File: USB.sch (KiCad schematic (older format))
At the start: 4 parts, among them J2 USB_B_Micro, U2 USBLC6-2SC6

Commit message: a
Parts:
- C15: footprint (none) -> Capacitor_SMD:C_0603_1608Metric
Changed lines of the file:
@@
 F 0 "C15" H 5365 3296 50  0000 L CNN
 F 1 "C" H 5365 3205 50  0000 L CNN
-F 2 "" H 5288 3100 50  0001 C CNN
+F 2 "Capacitor_SMD:C_0603_1608Metric" H 5288 3100 50  0001 C CNN
 F 3 "~" H 5250 3250 50  0001 C CNN
 	1    5250 3250

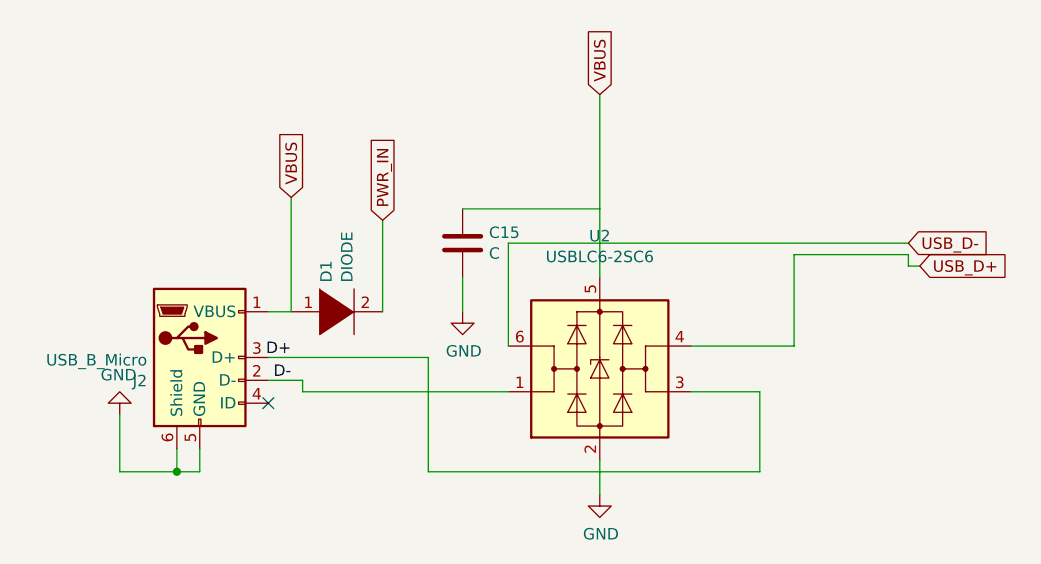
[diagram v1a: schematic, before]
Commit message: finish board
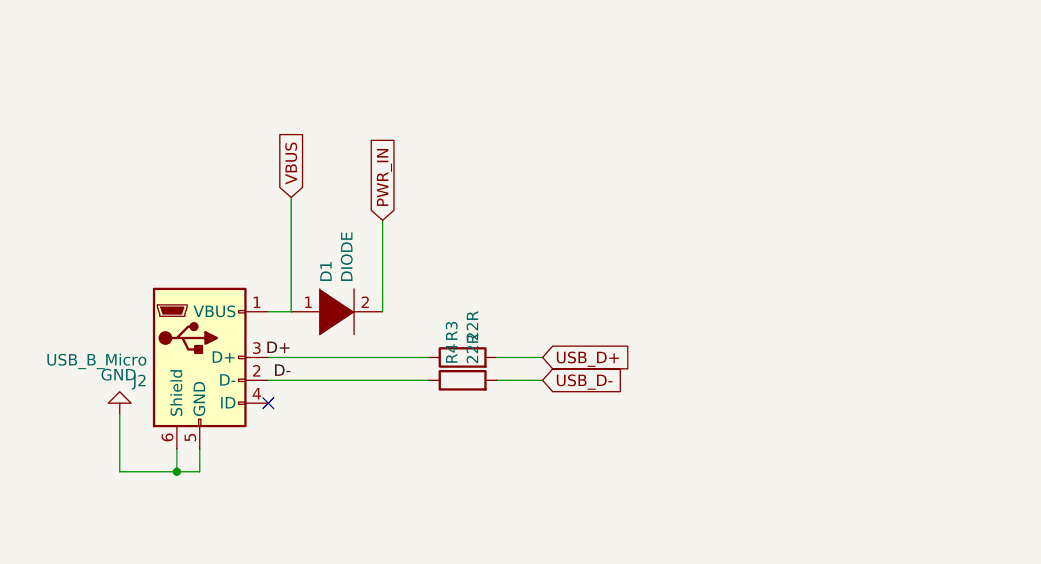
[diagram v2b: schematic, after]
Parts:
- removed C15: C, Capacitor_SMD:C_0603_1608Metric, symbol Device:C
- removed U2: USBLC6-2SC6, Package_TO_SOT_SMD:SOT-23-6, symbol Power_Protection:USBLC6-2SC6
- added R3, R4: 22R, Resistor_SMD:R_0603_1608Metric_Pad1.05x0.95mm_HandSolder, symbol Device:R
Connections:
- net D+: now also R3.1
- net D-: now also R4.1
- net USB_D+: now also R3.2
- net USB_D-: now also R4.2
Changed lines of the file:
@@
 Comment4 ""
 $EndDescr
-$Comp
-L Power_Protection:USBLC6-2SC6 U?
-U 1 1 5F5427BF
-P 5850 3800
-AR Path="/5F5427BF" Ref="U?"  Part="1"
-AR Path="/5F2F6324/5F5427BF" Ref="U?"  Part="1"
-AR Path="/5F53A524/5F5427BF" Ref="U2"  Part="1"
-AR Path="/5F584BC5/5F5427BF" Ref="U?"  Part="1"
-AR Path="/5FD47887/5F5427BF" Ref="U?"  Part="1"
-F 0 "U2" H 5850 4381 50  0000 C CNN
-F 1 "USBLC6-2SC6" H 5850 4290 50  0000 C CNN
-F 2 "Package_TO_SOT_SMD:SOT-23-6" H 5850 3300 50  0001 C CNN
-F 3 "https://www.st.com/resource/en/datasheet/usblc6-2.pdf" H 6050 4150 50  0001 C CNN
-	1    5850 3800
-	1    0    0    -1
-$EndComp
 Wire Wire Line
 	4100 4150 4100 4250
@@
 $EndComp
 NoConn ~ 4400 3950
-Wire Wire Line
-	4550 3850 4550 3900
-Wire Wire Line
-	4550 3850 4400 3850
 Text Label 4500 3750 2    50   ~ 0
 D+
@@
 D-
 Wire Wire Line
-	4550 3900 5450 3900
-Wire Wire Line
-	5100 3750 5100 4250
-Wire Wire Line
-	5100 4250 6550 4250
-Wire Wire Line
-	6550 4250 6550 3900
-Wire Wire Line
-	6550 3900 6250 3900
-Wire Wire Line
 	4400 3750 5100 3750
-Wire Wire Line
-	6250 3700 6700 3700
-Wire Wire Line
-	6700 3700 6700 3300
-Wire Wire Line
-	6700 3300 7200 3300
-Wire Wire Line
-	5450 3700 5450 3250
-Wire Wire Line
-	5450 3250 7200 3250
-Wire Wire Line
-	5850 3400 5850 3100
-Wire Wire Line
-	5850 4200 5850 4350
-$Comp
-L power:GND #PWR?
-U 1 1 5F5427E0
-P 5850 4350
-AR Path="/5F2F6324/5F5427E0" Ref="#PWR?"  Part="1"
-AR Path="/5F5427E0" Ref="#PWR?"  Part="1"
-AR Path="/5F53A524/5F5427E0" Ref="#PWR0112"  Part="1"
-AR Path="/5F584BC5/5F5427E0" Ref="#PWR?"  Part="1"
-AR Path="/5FD47887/5F5427E0" Ref="#PWR?"  Part="1"
-F 0 "#PWR0112" H 5850 4100 50  0001 C CNN
-F 1 "GND" H 5855 4177 50  0000 C CNN
-F 2 "" H 5850 4350 50  0001 C CNN
-F 3 "" H 5850 4350 50  0001 C CNN
-	1    5850 4350
-	1    0    0    -1
-$EndComp
-Wire Wire Line
-	7250 3350 7200 3350
-Wire Wire Line
-	7200 3350 7200 3300
-$Comp
-L Device:C C?
-U 1 1 5F5427E8
-P 5250 3250
-AR Path="/5F2F6324/5F5427E8" Ref="C?"  Part="1"
-AR Path="/5F5427E8" Ref="C?"  Part="1"
-AR Path="/5F53A524/5F5427E8" Ref="C15"  Part="1"
-AR Path="/5F584BC5/5F5427E8" Ref="C?"  Part="1"
-AR Path="/5FD47887/5F5427E8" Ref="C?"  Part="1"
-F 0 "C15" H 5365 3296 50  0000 L CNN
-F 1 "C" H 5365 3205 50  0000 L CNN
-F 2 "Capacitor_SMD:C_0603_1608Metric" H 5288 3100 50  0001 C CNN
-F 3 "~" H 5250 3250 50  0001 C CNN
-	1    5250 3250
-	1    0    0    -1
-$EndComp
-Wire Wire Line
-	5250 3100 5850 3100
-Wire Wire Line
-	5250 3400 5250 3550
-$Comp
-L power:GND #PWR?
-U 1 1 5F5427F0
-P 5250 3550
-AR Path="/5F2F6324/5F5427F0" Ref="#PWR?"  Part="1"
-AR Path="/5F5427F0" Ref="#PWR?"  Part="1"
-AR Path="/5F53A524/5F5427F0" Ref="#PWR0113"  Part="1"
-AR Path="/5F584BC5/5F5427F0" Ref="#PWR?"  Part="1"
-AR Path="/5FD47887/5F5427F0" Ref="#PWR?"  Part="1"
-F 0 "#PWR0113" H 5250 3300 50  0001 C CNN
-F 1 "GND" H 5255 3377 50  0000 C CNN
-F 2 "" H 5250 3550 50  0001 C CNN
-F 3 "" H 5250 3550 50  0001 C CNN
-	1    5250 3550
-	1    0    0    -1
-$EndComp
 Wire Wire Line
 	4400 3550 4500 3550
@@
 	1    0    0    -1
 $EndComp
-Text GLabel 7200 3250 2    50   Input ~ 0
+Text GLabel 5600 3850 2    50   Input ~ 0
 USB_D-
-Text GLabel 7250 3350 2    50   Input ~ 0
+Text GLabel 5600 3750 2    50   Input ~ 0
 USB_D+
 $Comp
@@
 Text GLabel 4500 3050 1    50   Input ~ 0
 VBUS
+$Comp
+L Device:R R?
+U 1 1 5F59BCFB
+P 5250 3750
+AR Path="/5F41B667/5F59BCFB" Ref="R?"  Part="1"
+AR Path="/5F59BCFB" Ref="R?"  Part="1"
+AR Path="/5F5517E4/5F59BCFB" Ref="R?"  Part="1"
+AR Path="/5F5C31DE/5F59BCFB" Ref="R?"  Part="1"
+AR Path="/5F53A524/5F59BCFB" Ref="R3"  Part="1"
+F 0 "R3" H 5320 3796 50  0000 L CNN
+F 1 "22R" H 5320 3705 50  0000 L CNN
+F 2 "Resistor_SMD:R_0603_1608Metric_Pad1.05x0.95mm_HandSolder" V 5180 3750 50  0001 C CNN
+F 3 "~" H 5250 3750 50  0001 C CNN
+	1    5250 3750
+	0    -1   -1   0
+$EndComp
+$Comp
+L Device:R R?
+U 1 1 5F59BEBC
+P 5250 3850
+AR Path="/5F41B667/5F59BEBC" Ref="R?"  Part="1"
+AR Path="/5F59BEBC" Ref="R?"  Part="1"
+AR Path="/5F5517E4/5F59BEBC" Ref="R?"  Part="1"
+AR Path="/5F5C31DE/5F59BEBC" Ref="R?"  Part="1"
+AR Path="/5F53A524/5F59BEBC" Ref="R4"  Part="1"
+F 0 "R4" H 5320 3896 50  0000 L CNN
+F 1 "22R" H 5320 3805 50  0000 L CNN
+F 2 "Resistor_SMD:R_0603_1608Metric_Pad1.05x0.95mm_HandSolder" V 5180 3850 50  0001 C CNN
+F 3 "~" H 5250 3850 50  0001 C CNN
+	1    5250 3850
+	0    -1   -1   0
+$EndComp
 Wire Wire Line
-	5850 2600 5850 3100
-Text GLabel 5850 2600 1    50   Input ~ 0
-VBUS
+	4400 3850 5100 3850
+Wire Wire Line
+	5400 3750 5600 3750
+Wire Wire Line
+	5400 3850 5600 3850
 $EndSCHEMATC
